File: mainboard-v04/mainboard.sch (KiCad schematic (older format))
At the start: 0 parts

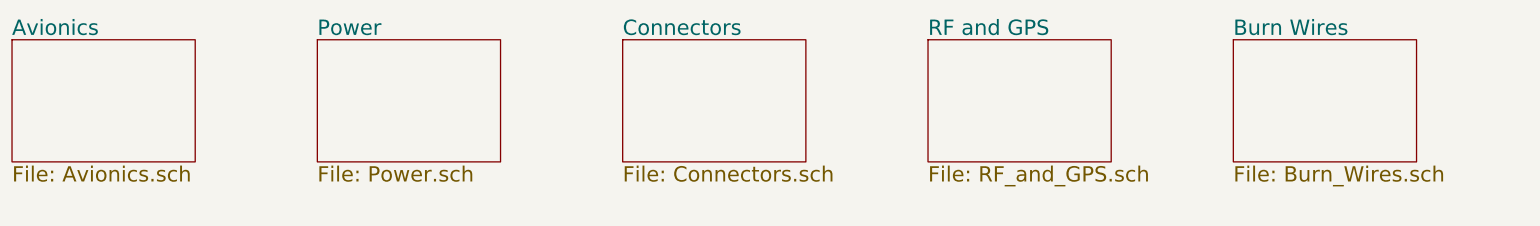
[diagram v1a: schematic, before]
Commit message: cleaned up v04
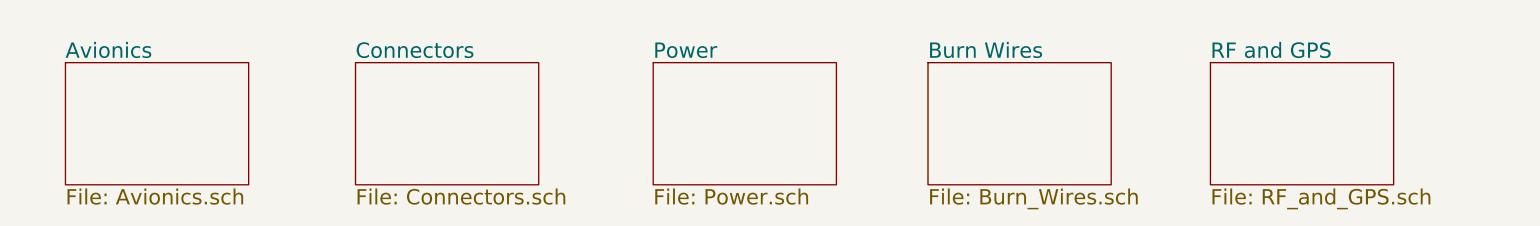
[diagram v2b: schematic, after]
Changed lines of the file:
@@
 Sheet 1 6
 Title "PyCubed Mainboard"
-Date "2020-01-08"
+Date "2020-02-10"
 Rev "v04"
-Comp ""
-Comment1 "Zac Manchester"
-Comment2 "Max Holliday"
+Comp "Max Holliday"
+Comment1 ""
+Comment2 ""
 Comment3 ""
 Comment4 ""
 $EndDescr
 $Sheet
-S 9000 2500 1200 800
+S 1350 2650 1200 800
+U 5CEC5A72
+F0 "Avionics" 100
+F1 "Avionics.sch" 100
+$EndSheet
+$Sheet
+S 3250 2650 1200 800
+U 5CEC60EB
+F0 "Connectors" 100
+F1 "Connectors.sch" 100
+$EndSheet
+$Sheet
+S 5200 2650 1200 800
+U 5CEC5DDE
+F0 "Power" 100
+F1 "Power.sch" 100
+$EndSheet
+$Sheet
+S 7000 2650 1200 800
 U 5CEC6476
 F0 "Burn Wires" 100
@@
 $EndSheet
 $Sheet
-S 7000 2500 1200 800
+S 8850 2650 1200 800
 U 5CEC6281
 F0 "RF and GPS" 100
 F1 "RF_and_GPS.sch" 100
 $EndSheet
-$Sheet
-S 5000 2500 1200 800
-U 5CEC60EB
-F0 "Connectors" 100
-F1 "Connectors.sch" 100
-$EndSheet
-$Sheet
-S 3000 2500 1200 800
-U 5CEC5DDE
-F0 "Power" 100
-F1 "Power.sch" 100
-$EndSheet
-$Sheet
-S 1000 2500 1200 800
-U 5CEC5A72
-F0 "Avionics" 100
-F1 "Avionics.sch" 100
-$EndSheet
 $EndSCHEMATC
